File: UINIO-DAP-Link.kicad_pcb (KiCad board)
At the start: 2 copper layers, 28 parts, among them J1 Conn_01x05_Male, J2 JTAG 输出, J3 JTAG_nTRST 跳线选择, J4 3.3V 跳线选择, J5 SWD 输入, J6 DAPLink 固件下载接口, J7 JTAG/SWD 下载接口, U1 STM32F103C8T6, Y1 Crystal_GND24

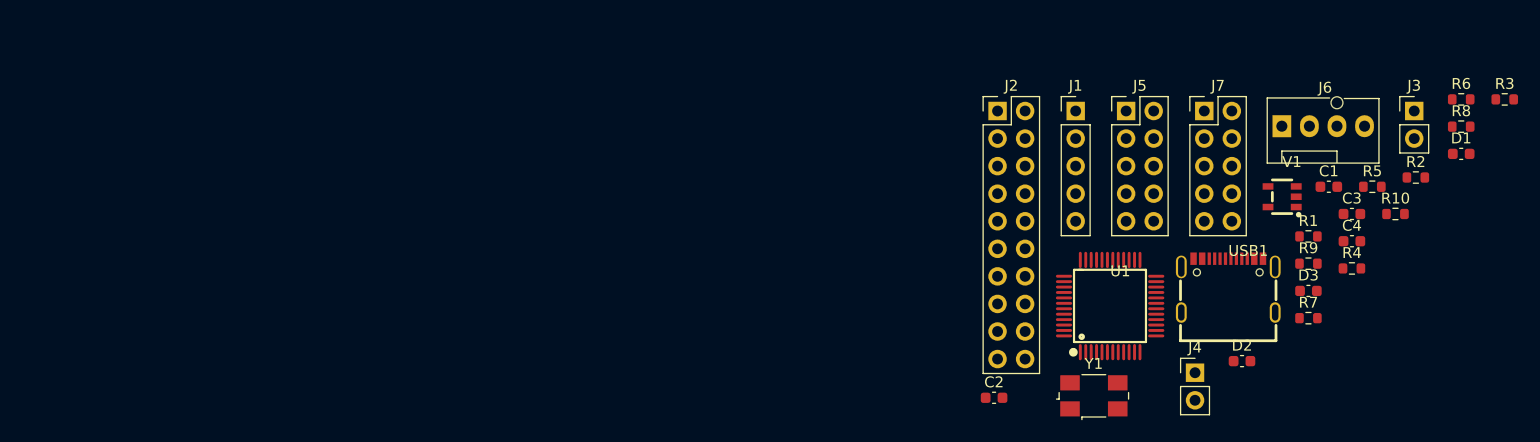
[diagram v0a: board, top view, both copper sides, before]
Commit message: Update PCB layout.
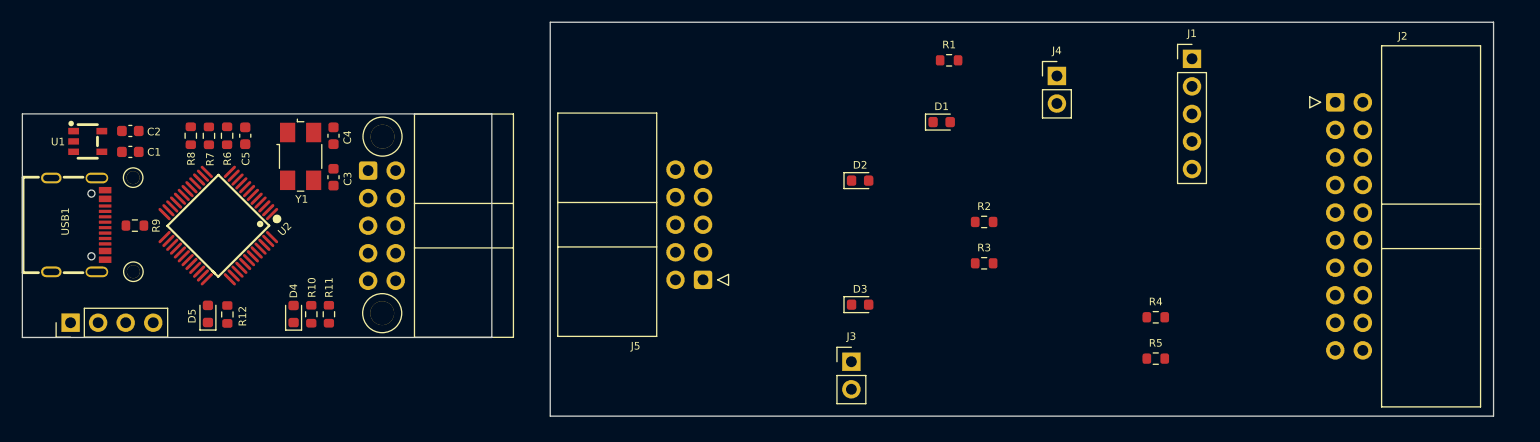
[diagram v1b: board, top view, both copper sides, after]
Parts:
- removed V1: ME6211, Uinio:SOT-23-5_L3.0-W1.7-P0.95-LS2.8-BR
- added C5: 0.1uF, Capacitor_SMD:C_0603_1608Metric, F.Cu at (52.3, 87.9)
- added D4: LED_Blue, LED_SMD:LED_0603_1608Metric, F.Cu at (56.8, 104.3)
- added D5: LED_Red, LED_SMD:LED_0603_1608Metric, F.Cu at (48.9, 104.3)
- added HOLE**: Hole-1mm, Uinio:Hole-1mm, F.Cu at (42.0, 91.7)
- added HOLE**: Hole-2mm, Uinio:Hole-2mm, F.Cu at (65.0, 104.2)
- added HOLE**: Hole-2mm, Uinio:Hole-2mm, F.Cu at (65.0, 88.0)
- added HOLE**: Hole-1mm, Uinio:Hole-1mm, F.Cu at (42.0, 100.4)
- added R11: 10K, Resistor_SMD:R_0603_1608Metric, F.Cu at (60.0, 104.3)
- added R12: 10K, Resistor_SMD:R_0603_1608Metric, F.Cu at (50.7, 104.3)
- added U2: STM32F103C8T6, Uinio:LQFP-48_L7.0-W7.0-P0.50-LS9.0, F.Cu at (49.8, 96.2)
- D1: value Blue LED -> LED_Red; footprint Capacitor_SMD:C_0603_1608Metric -> LED_SMD:LED_0603_1608Metric
- D2: value Blue LED -> LED_Blue; footprint Capacitor_SMD:C_0603_1608Metric -> LED_SMD:LED_0603_1608Metric
- D3: value BLUE LED -> LED_Blue; footprint Capacitor_SMD:C_0603_1608Metric -> LED_SMD:LED_0603_1608Metric
- J1: value Conn_01x05_Male -> 扩展板串口 & 电源输出
- J2: value JTAG 输出 -> 扩展板 JTAG 输出; footprint Connector_PinHeader_2.54mm:PinHeader_2x10_P2.54mm_Vertical -> Connector_IDC:IDC-Header_2x10_P2.54mm_Horizontal
- J5: value SWD 输入 -> 扩展板 SWD 输入; footprint Connector_PinHeader_2.54mm:PinHeader_2x05_P2.54mm_Vertical -> Connector_IDC:IDC-Header_2x05_P2.54mm_Horizontal
- J6: footprint Connector:FanPinHeader_1x04_P2.54mm_Vertical -> Connector_PinHeader_2.54mm:PinHeader_1x04_P2.54mm_Vertical
- J7: footprint Connector_PinHeader_2.54mm:PinHeader_2x05_P2.54mm_Vertical -> Connector_IDC:IDC-Header_2x05_P2.54mm_Horizontal
- U1: value STM32F103C8T6 -> ME6211; footprint Uinio:LQFP-48_L7.0-W7.0-P0.50-LS9.0 -> Uinio:SOT-23-5_L3.0-W1.7-P0.95-LS2.8-BR
- moved R8 117.1 mm to (47.3, 87.9), turned to -90 degrees
- moved R6 113.8 mm to (50.7, 87.9), turned to 90 degrees
- moved J6 113.1 mm to (36.2, 105.1), turned to 90 degrees
- moved C1 110.5 mm to (41.7, 89.4), turned to 180 degrees
- moved R9 108.2 mm to (42.2, 96.2)
- moved USB1 106.1 mm to (36.9, 96.1), turned to -90 degrees
- moved R7 102.7 mm to (49.0, 87.9), turned to 90 degrees
- moved R10 100.3 mm to (58.4, 104.3), turned to -90 degrees
- moved U1 95.4 mm to (37.8, 88.4), turned to 180 degrees
- moved C4 94.4 mm to (60.5, 87.9), turned to 90 degrees
- moved C3 93.9 mm to (60.5, 91.7), turned to -90 degrees
- moved C2 83.3 mm to (41.7, 87.4)
- moved J7 77.3 mm to (63.7, 91.1)
- moved Y1 76.4 mm to (57.4, 89.8), turned to -90 degrees
- moved J3 56.8 mm to (108.2, 108.7)
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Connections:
- R6 pad 1: /JTAG_nTRST -> Net-(C5-Pad1)
- R7 pad 1: /BOOT1 -> /JTAG_nTRST
- R7 pad 2: GND -> /VDD_3.3V
- R8 pad 1: Net-(R8-Pad1) -> /BOOT1
- R8 pad 2: /VDD_3.3V -> GND
- U1 pad 1: /VDD_3.3V -> /VDD_5V
- U1 pad 2: unconnected-(U1-Pad2) -> GND
- U1 pad 3: unconnected-(U1-Pad3) -> /VDD_5V
- U1 pad 4: unconnected-(U1-Pad4) -> Net-(C1-Pad2)
- U1 pad 5: Net-(U1-Pad5) -> /VDD_3.3V
- Y1 pad 1: Net-(U1-Pad6) -> Net-(U2-Pad6)
- Y1 pad 3: Net-(U1-Pad5) -> Net-(U2-Pad5)
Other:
- board outline added: 135.6 x 36.3 mm
